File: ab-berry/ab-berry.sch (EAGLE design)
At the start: 19 parts, among them U1 LM1117MPX-3.3/NOPB or AP2114H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

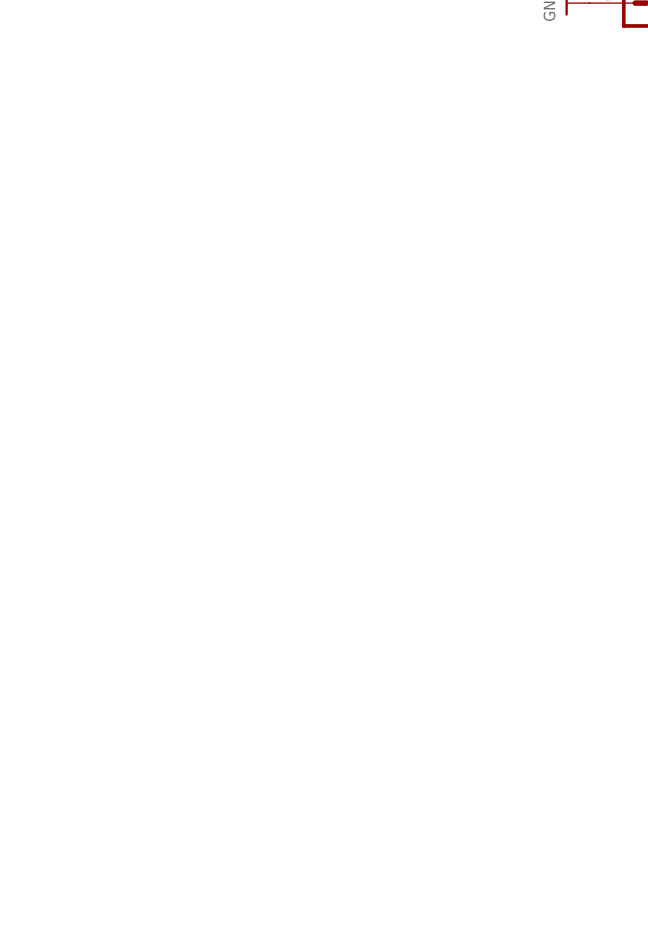
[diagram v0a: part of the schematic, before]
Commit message: wip
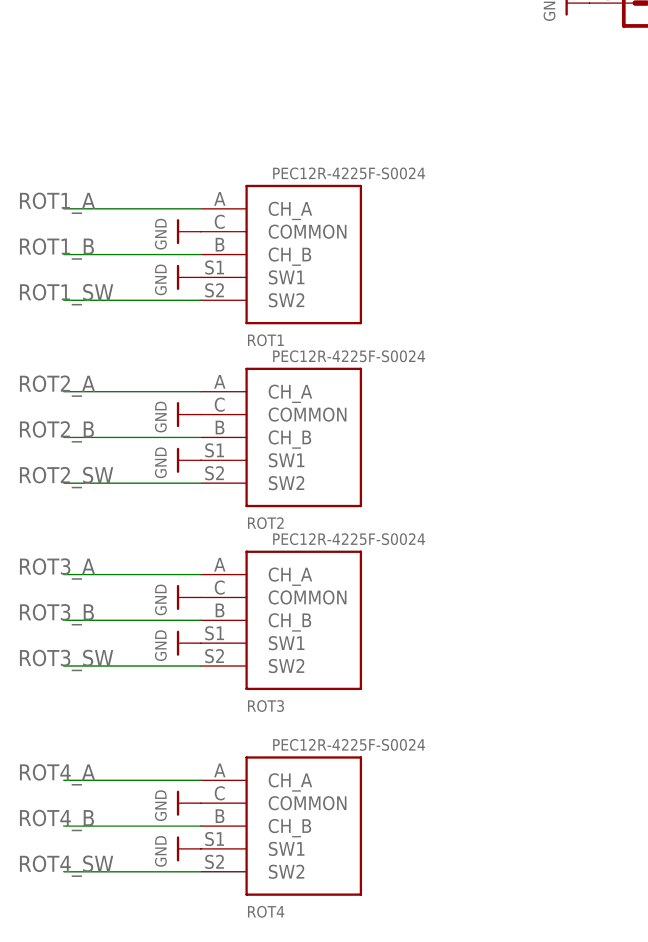
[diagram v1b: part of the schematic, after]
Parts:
- added ROT1, ROT2, ROT3, ROT4: PEC12R-4225F-S0024, keves:PEC11-4215K-S0024
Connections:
- new net ROT1_A: ROT1.CH_A
- new net ROT1_B: ROT1.CH_B
- new net ROT1_SW: ROT1.SW2
- new net ROT2_A: ROT2.CH_A
- new net ROT2_B: ROT2.CH_B
- new net ROT2_SW: ROT2.SW2
- new net ROT3_A: ROT3.CH_A
- new net ROT3_B: ROT3.CH_B
- new net ROT3_SW: ROT3.SW2
- new net ROT4_A: ROT4.CH_A
- new net ROT4_B: ROT4.CH_B
- new net ROT4_SW: ROT4.SW2
- net GND: now also ROT1.COMMON, ROT1.SW1, ROT2.COMMON, ROT2.SW1, ROT3.COMMON, ROT3.SW1, ROT4.COMMON, ROT4.SW1
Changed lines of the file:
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@@
 <layer number="121" name="sName" color="7" fill="1" visible="yes" active="yes"/>
 <layer number="122" name="_bPlace" color="7" fill="1" visible="yes" active="yes"/>
+<layer number="123" name="tTestmark" color="7" fill="1" visible="no" active="yes"/>
+<layer number="124" name="bTestmark" color="7" fill="1" visible="no" active="yes"/>
 <layer number="125" name="_tNames" color="7" fill="1" visible="yes" active="yes"/>
 <layer number="126" name="_bNames" color="7" fill="1" visible="yes" active="yes"/>
 <layer number="127" name="_tValues" color="7" fill="1" visible="yes" active="yes"/>
 <layer number="128" name="_bValues" color="7" fill="1" visible="yes" active="yes"/>
+<layer number="131" name="tAdjust" color="7" fill="1" visible="no" active="yes"/>
+<layer number="132" name="bAdjust" color="7" fill="1" visible="no" active="yes"/>
 <layer number="144" name="Drill_legend" color="7" fill="1" visible="yes" active="yes"/>
 <layer number="151" name="HeatSink" color="7" fill="1" visible="yes" active="yes"/>
 <layer number="152" name="_bDocu" color="7" fill="1" visible="yes" active="yes"/>
+<layer number="199" name="Contour" color="7" fill="1" visible="yes" active="yes"/>
 <layer number="200" name="200bmp" color="1" fill="10" visible="yes" active="yes"/>
 <layer number="201" name="201bmp" color="7" fill="1" visible="yes" active="yes"/>
@@
 <layer number="207" name="207bmp" color="8" fill="10" visible="yes" active="yes"/>
 <layer number="208" name="208bmp" color="9" fill="10" visible="yes" active="yes"/>
+<layer number="209" name="209bmp" color="7" fill="1" visible="no" active="yes"/>
+<layer number="210" name="210bmp" color="7" fill="1" visible="no" active="yes"/>
+<layer number="211" name="211bmp" color="7" fill="1" visible="no" active="yes"/>
+<layer number="212" name="212bmp" color="7" fill="1" visible="no" active="yes"/>
+<layer number="213" name="213bmp" color="7" fill="1" visible="no" active="yes"/>
+<layer number="214" name="214bmp" color="7" fill="1" visible="no" active="yes"/>
+<layer number="215" name="215bmp" color="7" fill="1" visible="no" active="yes"/>
+<layer number="216" name="216bmp" color="7" fill="1" visible="no" active="yes"/>
+<layer number="217" name="217bmp" color="18" fill="1" visible="no" active="no"/>
+<layer number="218" name="218bmp" color="19" fill="1" visible="no" active="no"/>
+<layer number="219" name="219bmp" color="20" fill="1" visible="no" active="no"/>
+<layer number="220" name="220bmp" color="21" fill="1" visible="no" active="no"/>
+<layer number="221" name="221bmp" color="22" fill="1" visible="no" active="no"/>
+<layer number="222" name="222bmp" color="23" fill="1" visible="no" active="no"/>
+<layer number="223" name="223bmp" color="24" fill="1" visible="no" active="no"/>
+<layer number="224" name="224bmp" color="25" fill="1" visible="no" active="no"/>
 <layer number="231" name="Eagle3D_PG1" color="14" fill="1" visible="yes" active="yes"/>
 <layer number="232" name="Eagle3D_PG2" color="14" fill="2" visible="yes" active="yes"/>
@@
 <part name="R5" library="microbuilder" deviceset="RESISTOR" device="0603" value="330"/>
 <part name="U$14" library="microbuilder" deviceset="GND" device=""/>
+<part name="ROT1" library="keves" deviceset="PEC11-4215K-S0024" device="" value="PEC12R-4225F-S0024"/>
+<part name="U$16" library="microbuilder" deviceset="GND" device=""/>
+<part name="U$17" library="microbuilder" deviceset="GND" device=""/>
+<part name="ROT2" library="keves" deviceset="PEC11-4215K-S0024" device="" value="PEC12R-4225F-S0024"/>
+<part name="U$15" library="microbuilder" deviceset="GND" device=""/>
+<part name="U$18" library="microbuilder" deviceset="GND" device=""/>
+<part name="ROT3" library="keves" deviceset="PEC11-4215K-S0024" device="" value="PEC12R-4225F-S0024"/>
+<part name="U$19" library="microbuilder" deviceset="GND" device=""/>
+<part name="U$20" library="microbuilder" deviceset="GND" device=""/>
+<part name="ROT4" library="keves" deviceset="PEC11-4215K-S0024" device="" value="PEC12R-4225F-S0024"/>
+<part name="U$21" library="microbuilder" deviceset="GND" device=""/>
+<part name="U$22" library="microbuilder" deviceset="GND" device=""/>
 </parts>
 <sheets>
@@
 <instance part="R5" gate="G$1" x="-38.1" y="76.2" rot="R90"/>
 <instance part="U$14" gate="G$1" x="-38.1" y="55.88"/>
+<instance part="ROT1" gate="G$1" x="-50.8" y="5.08"/>
+<instance part="U$16" gate="G$1" x="-63.5" y="7.62" rot="R270"/>
+<instance part="U$17" gate="G$1" x="-63.5" y="2.54" rot="R270"/>
+<instance part="ROT2" gate="G$1" x="-50.8" y="-15.24"/>
+<instance part="U$15" gate="G$1" x="-63.5" y="-12.7" rot="R270"/>
+<instance part="U$18" gate="G$1" x="-63.5" y="-17.78" rot="R270"/>
+<instance part="ROT3" gate="G$1" x="-50.8" y="-35.56"/>
+<instance part="U$19" gate="G$1" x="-63.5" y="-33.02" rot="R270"/>
+<instance part="U$20" gate="G$1" x="-63.5" y="-38.1" rot="R270"/>
+<instance part="ROT4" gate="G$1" x="-50.8" y="-58.42"/>
+<instance part="U$21" gate="G$1" x="-63.5" y="-55.88" rot="R270"/>
+<instance part="U$22" gate="G$1" x="-63.5" y="-60.96" rot="R270"/>
 </instances>
 <busses>
@@
 <wire x1="-58.42" y1="76.2" x2="-58.42" y2="73.66" width="0.1524" layer="91"/>
 <junction x="-58.42" y="73.66"/>
+</segment>
+<segment>
+<pinref part="ROT1" gate="G$1" pin="COMMON"/>
+<pinref part="U$16" gate="G$1" pin="GND"/>
+</segment>
+<segment>
+<pinref part="ROT1" gate="G$1" pin="SW1"/>
+<pinref part="U$17" gate="G$1" pin="GND"/>
+</segment>
+<segment>
+<pinref part="ROT2" gate="G$1" pin="COMMON"/>
+<pinref part="U$15" gate="G$1" pin="GND"/>
+</segment>
+<segment>
+<pinref part="ROT2" gate="G$1" pin="SW1"/>
+<pinref part="U$18" gate="G$1" pin="GND"/>
+</segment>
+<segment>
+<pinref part="ROT3" gate="G$1" pin="COMMON"/>
+<pinref part="U$19" gate="G$1" pin="GND"/>
+</segment>
+<segment>
+<pinref part="ROT3" gate="G$1" pin="SW1"/>
+<pinref part="U$20" gate="G$1" pin="GND"/>
+</segment>
+<segment>
+<pinref part="ROT4" gate="G$1" pin="COMMON"/>
+<pinref part="U$21" gate="G$1" pin="GND"/>
+</segment>
+<segment>
+<pinref part="ROT4" gate="G$1" pin="SW1"/>
+<pinref part="U$22" gate="G$1" pin="GND"/>
 </segment>
 </net>
@@
 </segment>
 </net>
+<net name="ROT1_A" class="0">
+<segment>
+<pinref part="ROT1" gate="G$1" pin="CH_A"/>
+<wire x1="-60.96" y1="10.16" x2="-76.2" y2="10.16" width="0.1524" layer="91"/>
+<label x="-81.28" y="10.16" size="1.778" layer="95"/>
+</segment>
+</net>
+<net name="ROT1_B" class="0">
+<segment>
+<pinref part="ROT1" gate="G$1" pin="CH_B"/>
+<wire x1="-60.96" y1="5.08" x2="-76.2" y2="5.08" width="0.1524" layer="91"/>
+<label x="-81.28" y="5.08" size="1.778" layer="95"/>
+</segment>
+</net>
+<net name="ROT1_SW" class="0">
+<segment>
+<pinref part="ROT1" gate="G$1" pin="SW2"/>
+<wire x1="-60.96" y1="0" x2="-76.2" y2="0" width="0.1524" layer="91"/>
+<label x="-81.28" y="0" size="1.778" layer="95"/>
+</segment>
+</net>
+<net name="ROT2_A" class="0">
+<segment>
+<pinref part="ROT2" gate="G$1" pin="CH_A"/>
+<wire x1="-60.96" y1="-10.16" x2="-76.2" y2="-10.16" width="0.1524" layer="91"/>
+<label x="-81.28" y="-10.16" size="1.778" layer="95"/>
+</segment>
+</net>
+<net name="ROT2_B" class="0">
+<segment>
+<pinref part="ROT2" gate="G$1" pin="CH_B"/>
+<wire x1="-60.96" y1="-15.24" x2="-76.2" y2="-15.24" width="0.1524" layer="91"/>
+<label x="-81.28" y="-15.24" size="1.778" layer="95"/>
+</segment>
+</net>
+<net name="ROT2_SW" class="0">
+<segment>
+<pinref part="ROT2" gate="G$1" pin="SW2"/>
+<wire x1="-60.96" y1="-20.32" x2="-76.2" y2="-20.32" width="0.1524" layer="91"/>
+<label x="-81.28" y="-20.32" size="1.778" layer="95"/>
+</segment>
+</net>
+<net name="ROT3_A" class="0">
+<segment>
+<pinref part="ROT3" gate="G$1" pin="CH_A"/>
+<wire x1="-60.96" y1="-30.48" x2="-76.2" y2="-30.48" width="0.1524" layer="91"/>
+<label x="-81.28" y="-30.48" size="1.778" layer="95"/>
+</segment>
+</net>
+<net name="ROT3_B" class="0">
+<segment>
+<pinref part="ROT3" gate="G$1" pin="CH_B"/>
+<wire x1="-60.96" y1="-35.56" x2="-76.2" y2="-35.56" width="0.1524" layer="91"/>
+<label x="-81.28" y="-35.56" size="1.778" layer="95"/>
+</segment>
+</net>
+<net name="ROT3_SW" class="0">
+<segment>
+<pinref part="ROT3" gate="G$1" pin="SW2"/>
+<wire x1="-60.96" y1="-40.64" x2="-76.2" y2="-40.64" width="0.1524" layer="91"/>
+<label x="-81.28" y="-40.64" size="1.778" layer="95"/>
+</segment>
+</net>
+<net name="ROT4_A" class="0">
+<segment>
+<pinref part="ROT4" gate="G$1" pin="CH_A"/>
+<wire x1="-60.96" y1="-53.34" x2="-76.2" y2="-53.34" width="0.1524" layer="91"/>
+<label x="-81.28" y="-53.34" size="1.778" layer="95"/>
+</segment>
+</net>
+<net name="ROT4_B" class="0">
+<segment>
+<pinref part="ROT4" gate="G$1" pin="CH_B"/>
+<wire x1="-60.96" y1="-58.42" x2="-76.2" y2="-58.42" width="0.1524" layer="91"/>
+<label x="-81.28" y="-58.42" size="1.778" layer="95"/>
+</segment>
+</net>
+<net name="ROT4_SW" class="0">
+<segment>
+<pinref part="ROT4" gate="G$1" pin="SW2"/>
+<wire x1="-60.96" y1="-63.5" x2="-76.2" y2="-63.5" width="0.1524" layer="91"/>
+<label x="-81.28" y="-63.5" size="1.778" layer="95"/>
+</segment>
+</net>

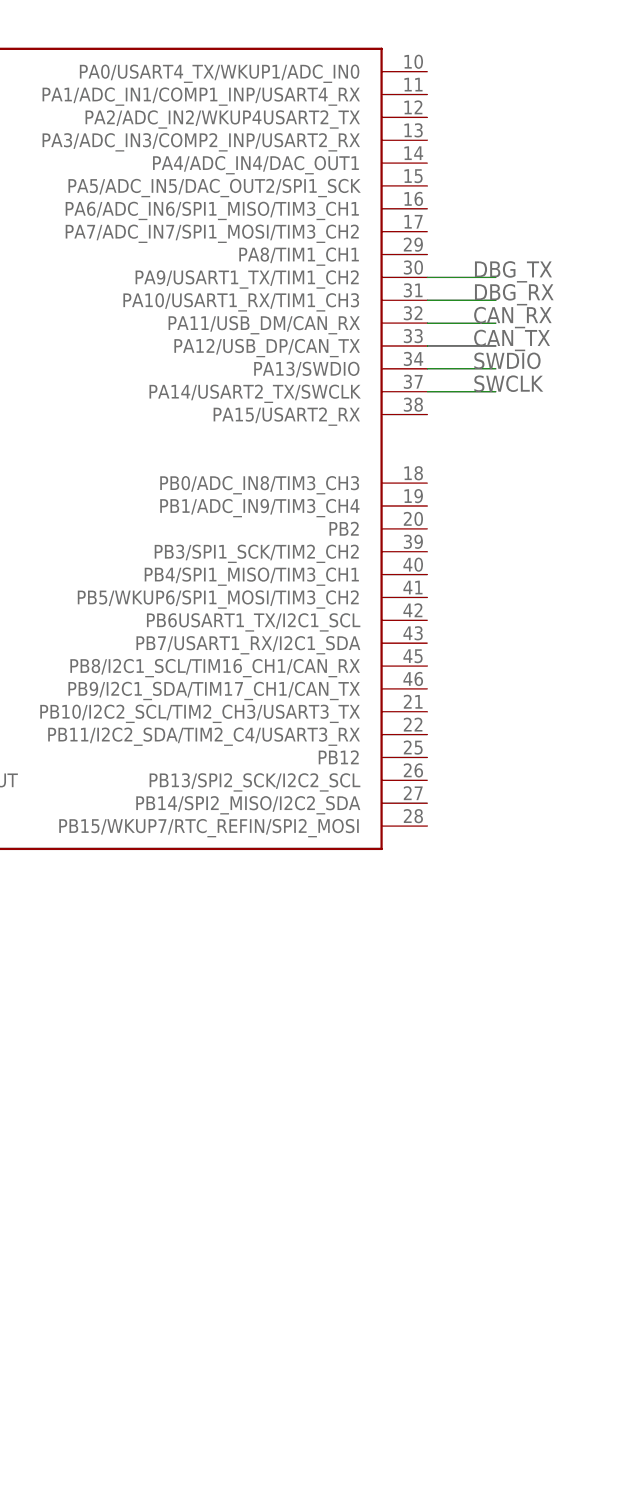
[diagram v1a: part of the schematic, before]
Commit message: wip
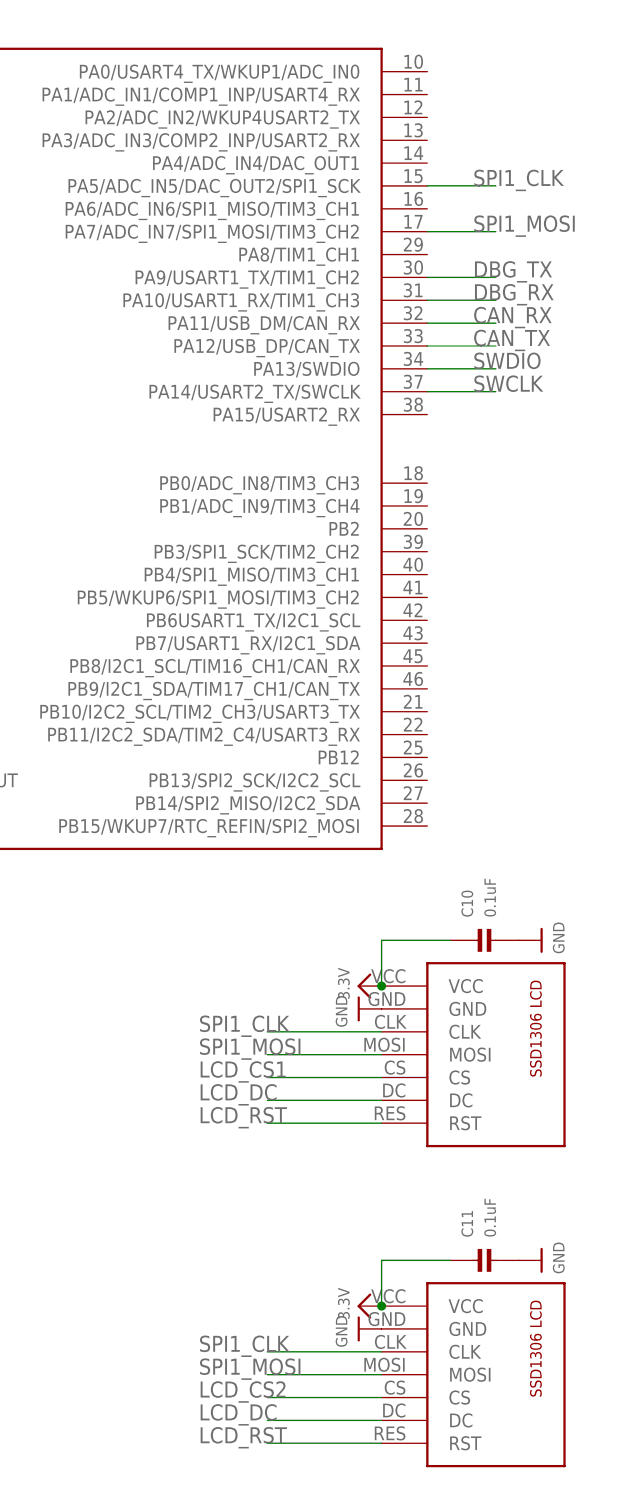
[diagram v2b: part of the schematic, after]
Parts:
- added C10, C11: 0.1uF, microbuilder:CAP_CERAMIC0603
- added LCD1, LCD2: SSD1306-7PIN, keves:SSD1306-7PIN
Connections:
- new net LCD_CS1: LCD1.CS
- new net LCD_CS2: LCD2.CS
- new net LCD_DC: LCD1.DC, LCD2.DC
- new net LCD_RST: LCD1.RST, LCD2.RST
- new net SPI1_CLK: LCD1.CLK, LCD2.CLK, STM32F072CBT6.PA5/ADC_IN5/DAC_OUT2/SPI1_SCK
- new net SPI1_MOSI: LCD1.MOSI, LCD2.MOSI, STM32F072CBT6.PA7/ADC_IN7/SPI1_MOSI/TIM3_CH2
- net 3.3V: now also C10.P$1, C11.P$1, LCD1.VCC, LCD2.VCC
- net GND: now also C10.P$2, C11.P$2, LCD1.GND, LCD2.GND
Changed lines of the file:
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@@
 <part name="U$21" library="microbuilder" deviceset="GND" device=""/>
 <part name="U$22" library="microbuilder" deviceset="GND" device=""/>
+<part name="LCD1" library="keves" deviceset="SSD1306-7PIN" device=""/>
+<part name="C10" library="microbuilder" deviceset="CAP_CERAMIC" device="0603" value="0.1uF"/>
+<part name="U$23" library="microbuilder" deviceset="GND" device=""/>
+<part name="U$24" library="microbuilder" deviceset="GND" device=""/>
+<part name="U$25" library="microbuilder" deviceset="3.3V" device=""/>
+<part name="LCD2" library="keves" deviceset="SSD1306-7PIN" device=""/>
+<part name="C11" library="microbuilder" deviceset="CAP_CERAMIC" device="0603" value="0.1uF"/>
+<part name="U$26" library="microbuilder" deviceset="GND" device=""/>
+<part name="U$27" library="microbuilder" deviceset="GND" device=""/>
+<part name="U$28" library="microbuilder" deviceset="3.3V" device=""/>
 </parts>
 <sheets>
@@
 <instance part="U$21" gate="G$1" x="-63.5" y="-55.88" rot="R270"/>
 <instance part="U$22" gate="G$1" x="-63.5" y="-60.96" rot="R270"/>
+<instance part="LCD1" gate="G$1" x="124.46" y="-20.32"/>
+<instance part="C10" gate="G$1" x="124.46" y="-10.16" rot="R90"/>
+<instance part="U$23" gate="G$1" x="129.54" y="-10.16" rot="R90"/>
+<instance part="U$24" gate="G$1" x="109.22" y="-17.78" rot="R270"/>
+<instance part="U$25" gate="G$1" x="109.22" y="-15.24" rot="R90"/>
+<instance part="LCD2" gate="G$1" x="124.46" y="-55.88"/>
+<instance part="C11" gate="G$1" x="124.46" y="-45.72" rot="R90"/>
+<instance part="U$26" gate="G$1" x="129.54" y="-45.72" rot="R90"/>
+<instance part="U$27" gate="G$1" x="109.22" y="-53.34" rot="R270"/>
+<instance part="U$28" gate="G$1" x="109.22" y="-50.8" rot="R90"/>
 </instances>
 <busses>
@@
 <pinref part="ROT4" gate="G$1" pin="SW1"/>
 <pinref part="U$22" gate="G$1" pin="GND"/>
+</segment>
+<segment>
+<pinref part="C10" gate="G$1" pin="P$2"/>
+<pinref part="U$23" gate="G$1" pin="GND"/>
+</segment>
+<segment>
+<pinref part="LCD1" gate="G$1" pin="GND"/>
+<pinref part="U$24" gate="G$1" pin="GND"/>
+</segment>
+<segment>
+<pinref part="C11" gate="G$1" pin="P$2"/>
+<pinref part="U$26" gate="G$1" pin="GND"/>
+</segment>
+<segment>
+<pinref part="LCD2" gate="G$1" pin="GND"/>
+<pinref part="U$27" gate="G$1" pin="GND"/>
 </segment>
 </net>
@@
 <junction x="-38.1" y="83.82"/>
 </segment>
+<segment>
+<pinref part="LCD1" gate="G$1" pin="VCC"/>
+<pinref part="U$25" gate="G$1" pin="3.3V"/>
+<pinref part="C10" gate="G$1" pin="P$1"/>
+<wire x1="119.38" y1="-10.16" x2="111.76" y2="-10.16" width="0.1524" layer="91"/>
+<wire x1="111.76" y1="-10.16" x2="111.76" y2="-15.24" width="0.1524" layer="91"/>
+<junction x="111.76" y="-15.24"/>
+</segment>
+<segment>
+<pinref part="LCD2" gate="G$1" pin="VCC"/>
+<pinref part="U$28" gate="G$1" pin="3.3V"/>
+<pinref part="C11" gate="G$1" pin="P$1"/>
+<wire x1="119.38" y1="-45.72" x2="111.76" y2="-45.72" width="0.1524" layer="91"/>
+<wire x1="111.76" y1="-45.72" x2="111.76" y2="-50.8" width="0.1524" layer="91"/>
+<junction x="111.76" y="-50.8"/>
+</segment>
 </net>
 <net name="SWDIO" class="0">
@@
 </segment>
 </net>
+<net name="SPI1_MOSI" class="0">
+<segment>
+<pinref part="LCD1" gate="G$1" pin="MOSI"/>
+<wire x1="111.76" y1="-22.86" x2="99.06" y2="-22.86" width="0.1524" layer="91"/>
+<label x="91.44" y="-22.86" size="1.778" layer="95"/>
+</segment>
+<segment>
+<pinref part="LCD2" gate="G$1" pin="MOSI"/>
+<wire x1="111.76" y1="-58.42" x2="99.06" y2="-58.42" width="0.1524" layer="91"/>
+<label x="91.44" y="-58.42" size="1.778" layer="95"/>
+</segment>
+<segment>
+<pinref part="STM32F072CBT6" gate="G$1" pin="PA7/ADC_IN7/SPI1_MOSI/TIM3_CH2"/>
+<wire x1="116.84" y1="68.58" x2="124.46" y2="68.58" width="0.1524" layer="91"/>
+<label x="121.92" y="68.58" size="1.778" layer="95"/>
+</segment>
+</net>
+<net name="LCD_CS1" class="0">
+<segment>
+<pinref part="LCD1" gate="G$1" pin="CS"/>
+<wire x1="111.76" y1="-25.4" x2="99.06" y2="-25.4" width="0.1524" layer="91"/>
+<label x="91.44" y="-25.4" size="1.778" layer="95"/>
+</segment>
+</net>
+<net name="LCD_DC" class="0">
+<segment>
+<pinref part="LCD1" gate="G$1" pin="DC"/>
+<wire x1="111.76" y1="-27.94" x2="99.06" y2="-27.94" width="0.1524" layer="91"/>
+<label x="91.44" y="-27.94" size="1.778" layer="95"/>
+</segment>
+<segment>
+<pinref part="LCD2" gate="G$1" pin="DC"/>
+<wire x1="111.76" y1="-63.5" x2="99.06" y2="-63.5" width="0.1524" layer="91"/>
+<label x="91.44" y="-63.5" size="1.778" layer="95"/>
+</segment>
+</net>
+<net name="LCD_RST" class="0">
+<segment>
+<pinref part="LCD1" gate="G$1" pin="RST"/>
+<wire x1="111.76" y1="-30.48" x2="99.06" y2="-30.48" width="0.1524" layer="91"/>
+<label x="91.44" y="-30.48" size="1.778" layer="95"/>
+</segment>
+<segment>
+<pinref part="LCD2" gate="G$1" pin="RST"/>
+<wire x1="111.76" y1="-66.04" x2="99.06" y2="-66.04" width="0.1524" layer="91"/>
+<label x="91.44" y="-66.04" size="1.778" layer="95"/>
+</segment>
+</net>
+<net name="SPI1_CLK" class="0">
+<segment>
+<pinref part="LCD1" gate="G$1" pin="CLK"/>
+<wire x1="111.76" y1="-20.32" x2="99.06" y2="-20.32" width="0.1524" layer="91"/>
+<label x="91.44" y="-20.32" size="1.778" layer="95"/>
+</segment>
+<segment>
+<pinref part="LCD2" gate="G$1" pin="CLK"/>
+<wire x1="111.76" y1="-55.88" x2="99.06" y2="-55.88" width="0.1524" layer="91"/>
+<label x="91.44" y="-55.88" size="1.778" layer="95"/>
+</segment>
+<segment>
+<pinref part="STM32F072CBT6" gate="G$1" pin="PA5/ADC_IN5/DAC_OUT2/SPI1_SCK"/>
+<wire x1="116.84" y1="73.66" x2="124.46" y2="73.66" width="0.1524" layer="91"/>
+<label x="121.92" y="73.66" size="1.778" layer="95"/>
+</segment>
+</net>
+<net name="LCD_CS2" class="0">
+<segment>
+<pinref part="LCD2" gate="G$1" pin="CS"/>
+<wire x1="111.76" y1="-60.96" x2="99.06" y2="-60.96" width="0.1524" layer="91"/>
+<label x="91.44" y="-60.96" size="1.778" layer="95"/>
+</segment>
+</net>
